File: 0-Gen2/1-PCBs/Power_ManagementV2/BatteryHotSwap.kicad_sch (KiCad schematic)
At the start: 43 parts, among them J3 Conn_01x04_Pin, K1 G5V-1 DC3, Q5 MCTL160N15Y-TP, Q6 MCTL160N15Y-TP, Q7 MCTL160N15Y-TP, U10 74LVC1G08, U11 74LVC1G08, U12 74LVC1G08, U13 74LVC1G08, U15 74AHC1G04, U16 74LVC1G08, U8 LM393DT, U9 LTC1255CS8-PBF

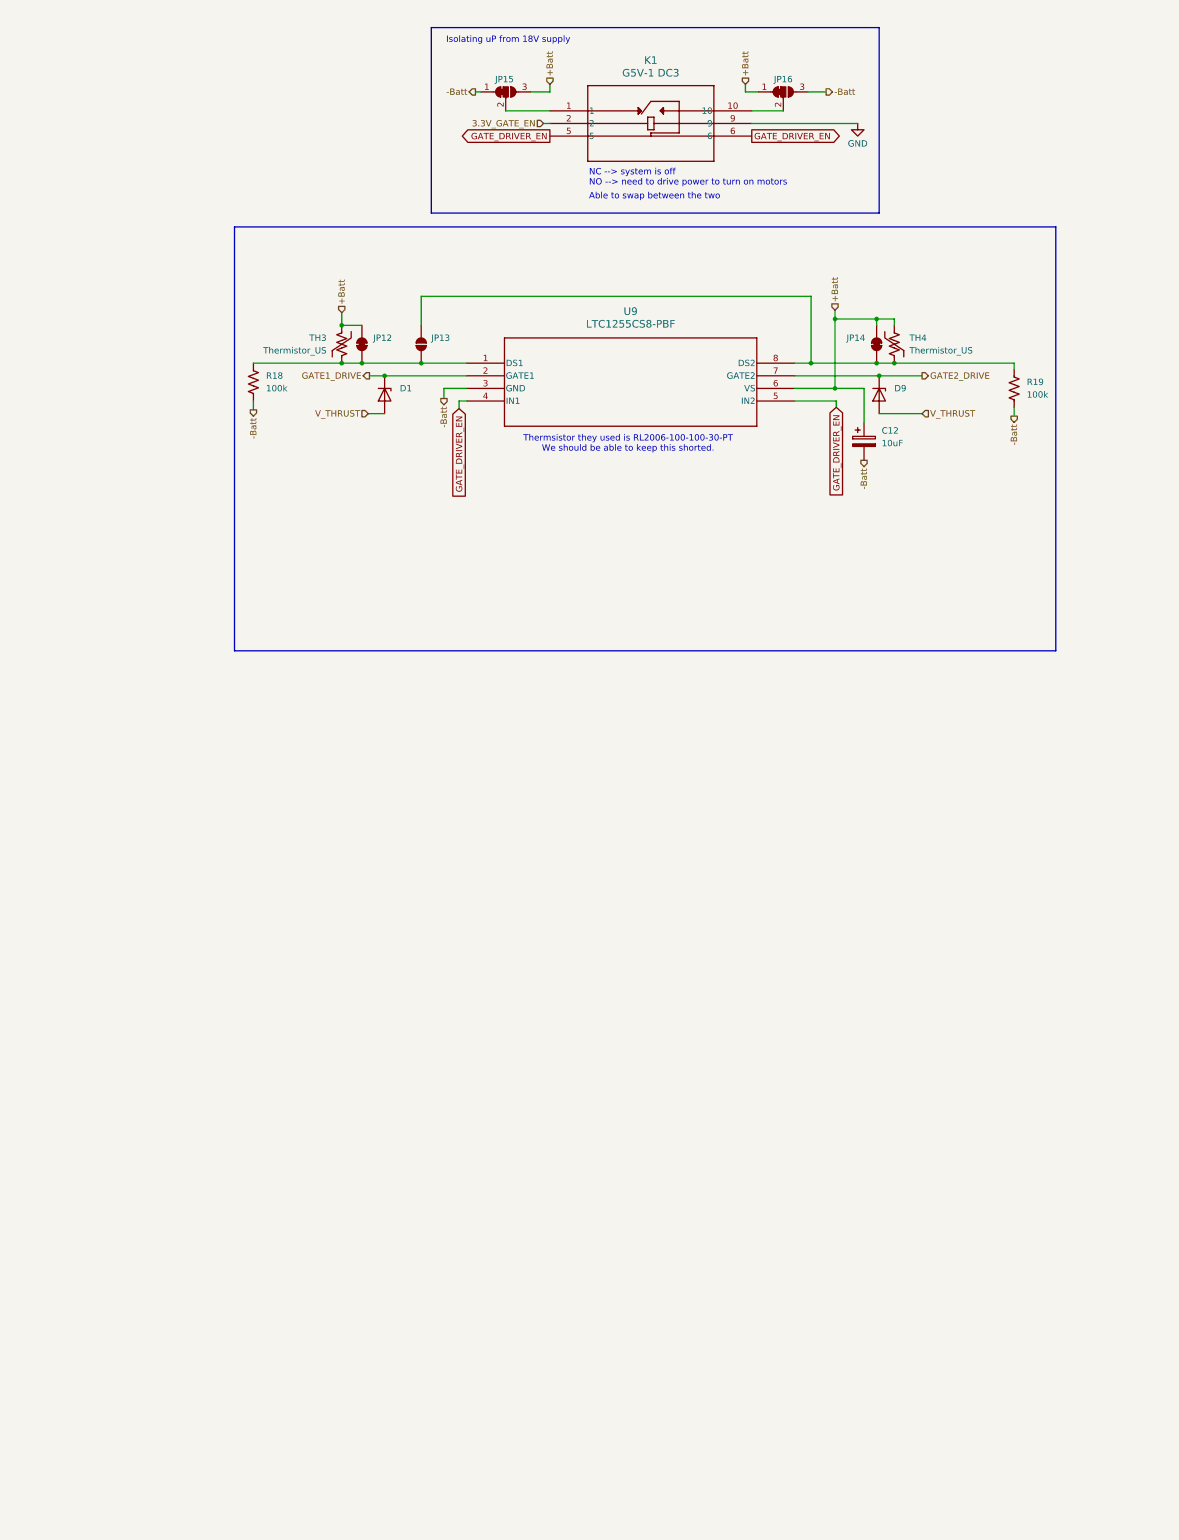
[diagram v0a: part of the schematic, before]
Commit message: progress distribution
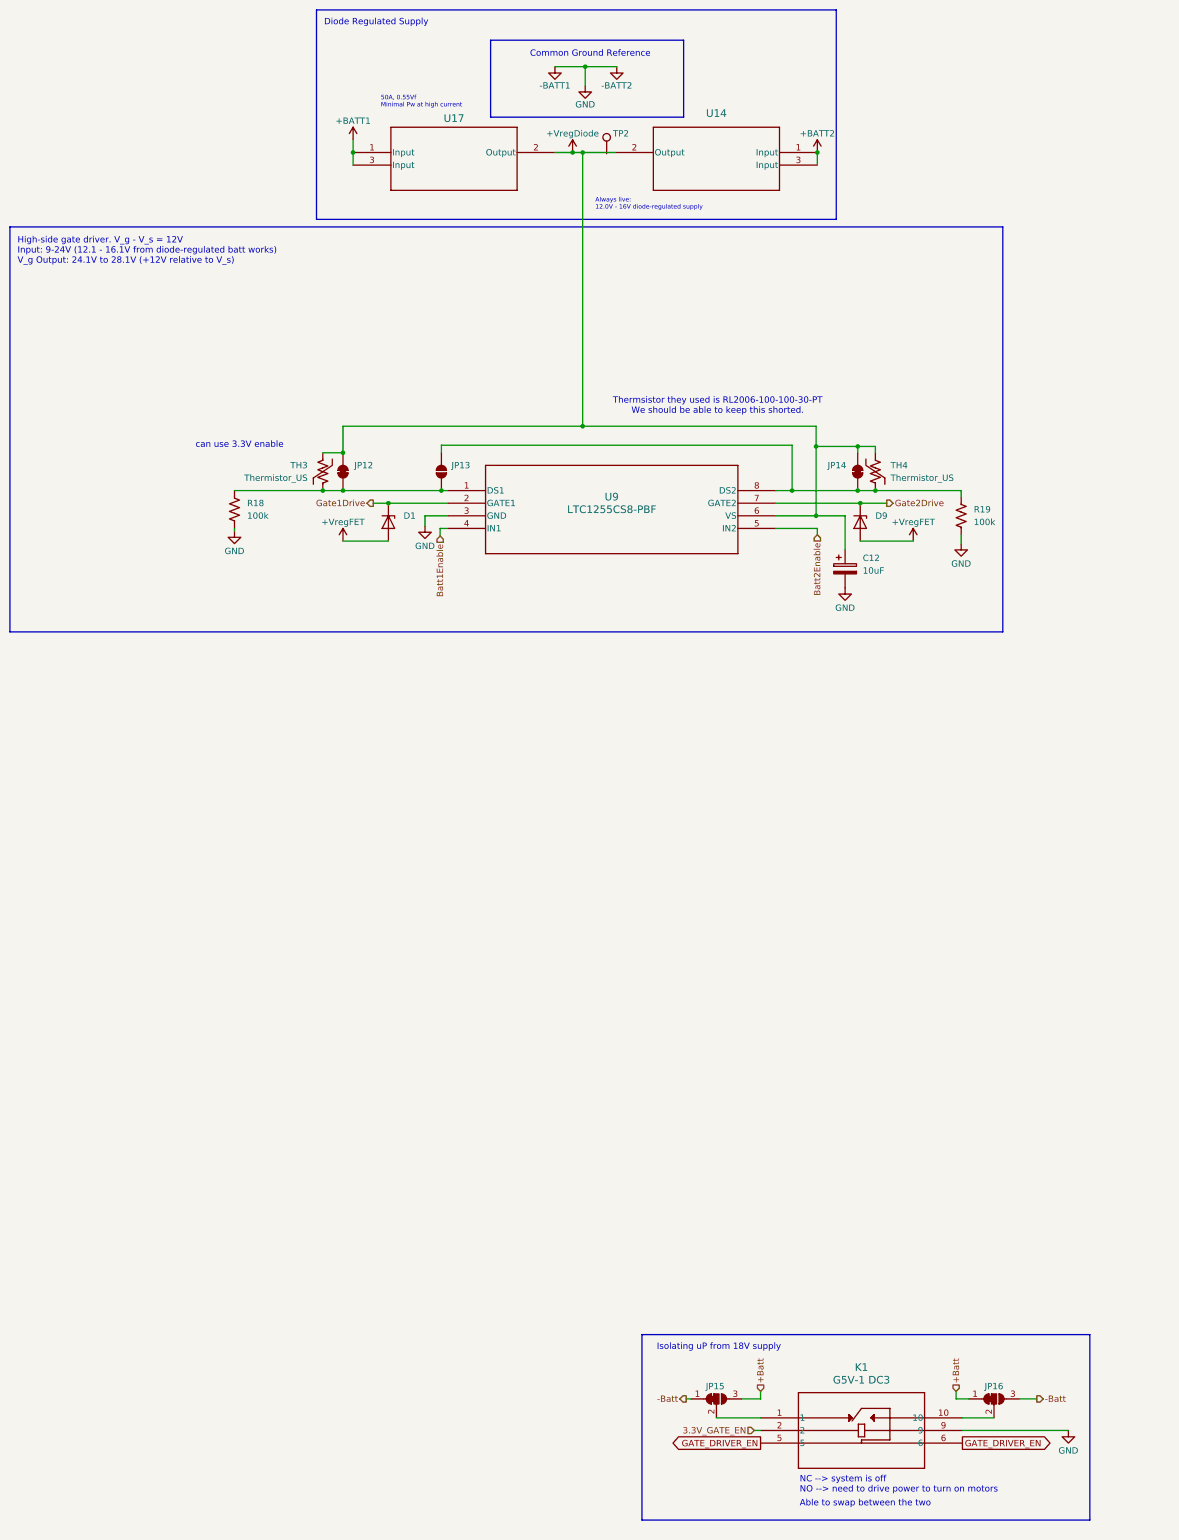
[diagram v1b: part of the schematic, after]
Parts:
- added TP2: DiodeRegSupply, TestPoint:TestPoint_Keystone_5019_Minature, symbol Connector:TestPoint
- added U14, U17: STPS5045SG-TR, Imported_Footprints:D2PAK_STM, symbol Imported_Symbols:STPS5045SG-TR
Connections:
- net -BATT2 is gone; now on net -BATT1: R5.2
- net GND is gone; now on net -BATT1: D10.1 (K), D11.1 (K), D12.1 (K), D13.1 (K), D14.1 (K), D15.1 (K), K1.9, U10.3 (GND), U11.3 (GND), U12.3 (GND), U13.3 (GND), U16.3 (GND), U8.4 (VCC-)
- net +BATT1: now also U17.1 (Input), U17.3 (Input)
- net +BATT2: now also U14.1 (Input), U14.3 (Input)
- net +Batt: no longer C12.1, JP12.2 (B), JP14.2 (B), TH3.1, TH4.1, U9.6 (VS)
- net -BATT1: now also C12.2, R18.1, R19.1, U9.3 (GND)
- net -Batt: no longer C12.2, R18.1, R19.1, U9.3 (GND)
- net GATE_DRIVER_EN: no longer U9.4 (IN1), U9.5 (IN2)
- net V_THRUST: no longer D1.2 (A), D9.2 (A)
- net GATE1_DRIVE renamed Gate1Drive
- net GATE2_DRIVE renamed Gate2Drive
- new net +VregDiode: C12.1, JP12.2 (B), JP14.2 (B), TH3.1, TH4.1, U14.2 (Output), U17.2 (Output), U9.6 (VS)
- new net +VregFET: D1.2 (A), D9.2 (A)
- new net Batt1Enable: U9.4 (IN1)
- new net Batt2Enable: U9.5 (IN2)
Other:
- note added: "50A, 0.55Vf Minimal Pw at high current"
- note added: "Always live: 12.0V - 16V diode-regulated supply"
- note added: "Common Ground Reference"
- note added: "Diode Regulated Supply"
- note added: "High-side gate driver. V_g - V_s = 12V Input: 9-24V (12.1 - 16.1V from diode-regulated batt works) V_g Output: 24.1V to 28.1V (+12V relative to V_s)"
- note added: "can use 3.3V enable"
- moved on the sheet: C12, D1, D9, JP12, JP13, JP14, JP15, JP16, K1, R18, R19, TH3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
